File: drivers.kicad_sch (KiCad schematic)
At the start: 61 parts, among them J12 Conn_01x06_Female, Q1 FQP30N06, Q2 FQP30N06, Q3 FQP30N06, Q4 FQP30N06, Q5 FQP30N06, Q6 FQP30N06

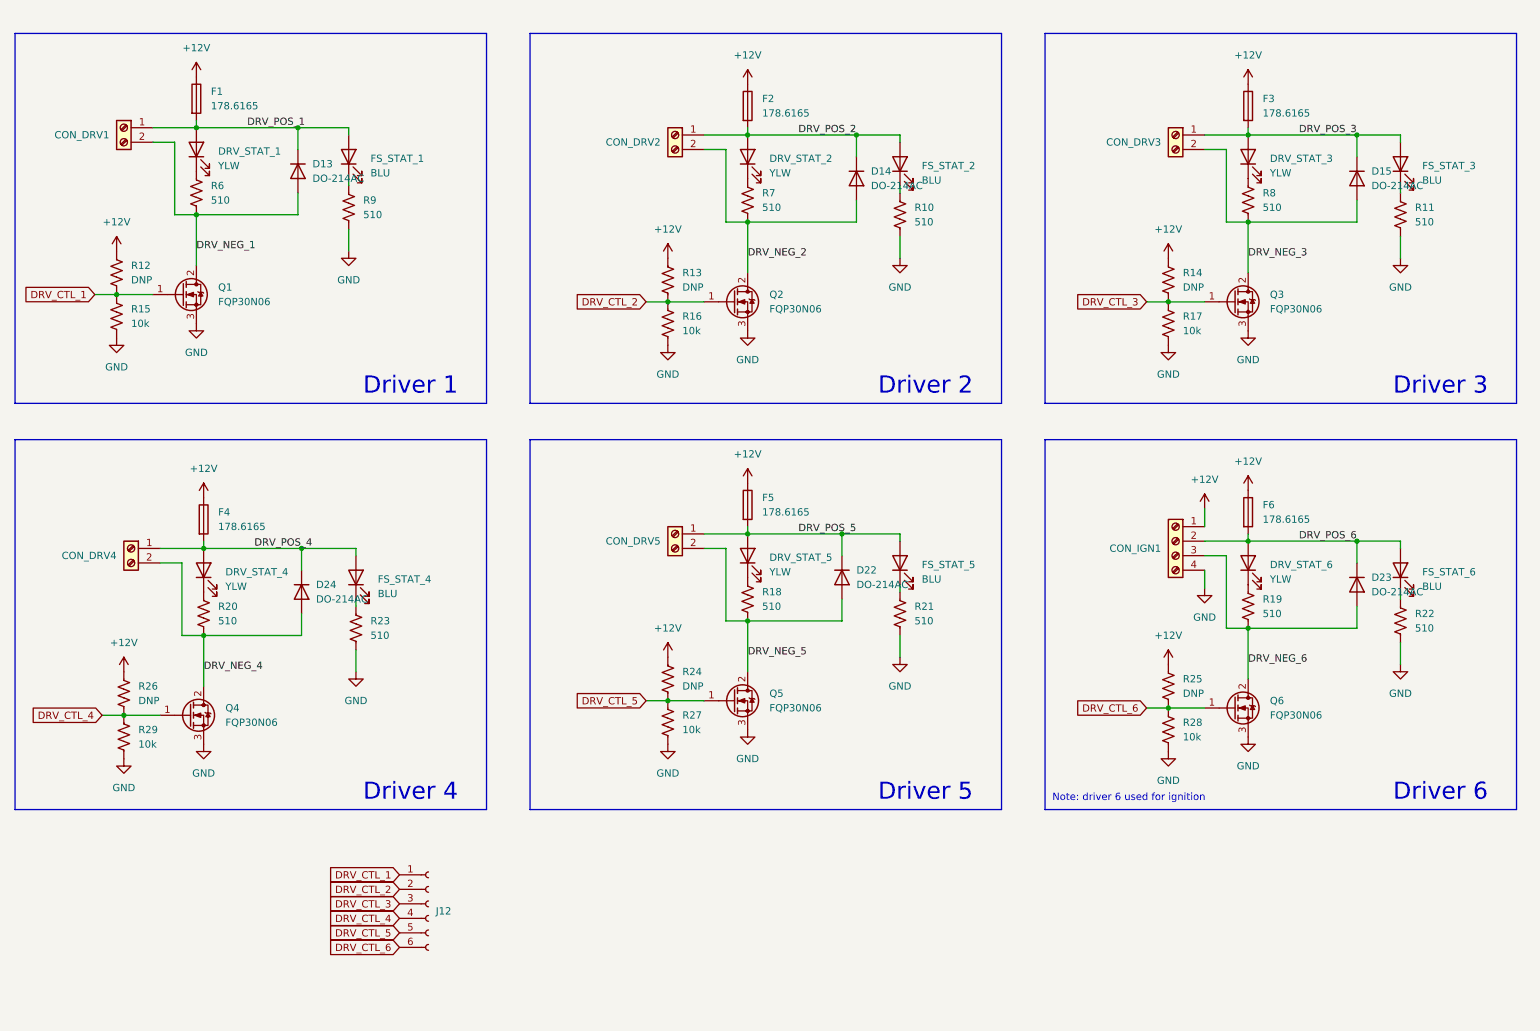
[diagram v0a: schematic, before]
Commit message: done schematiccing after design review
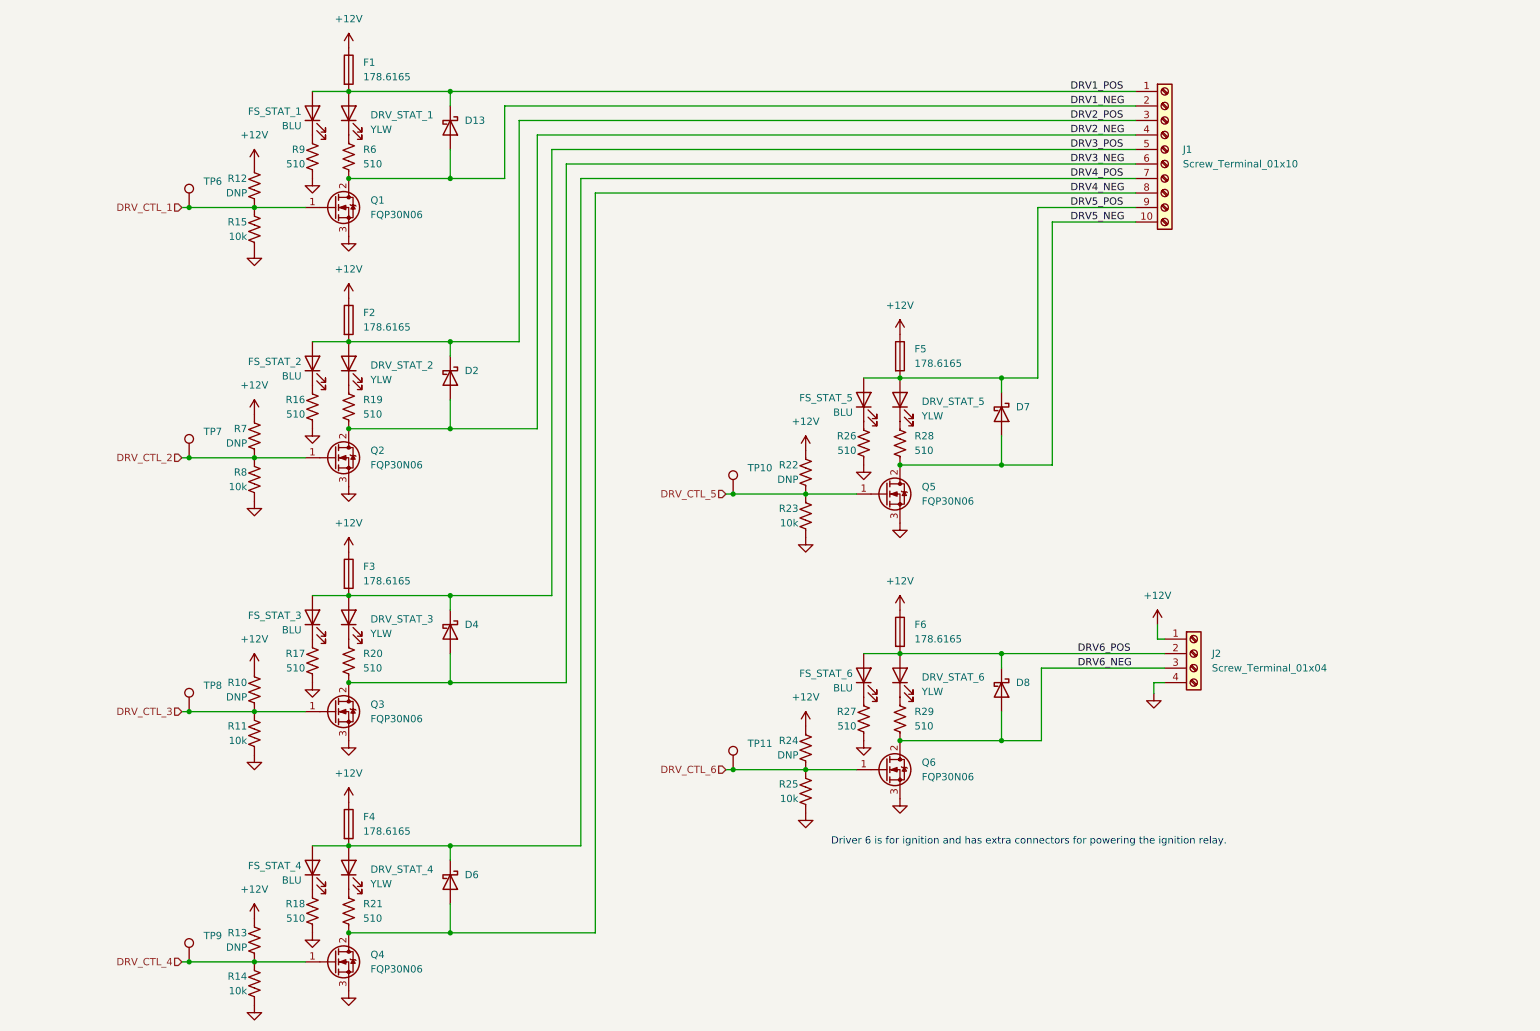
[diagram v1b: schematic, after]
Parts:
- removed CON_DRV1, CON_DRV2, CON_DRV3, CON_DRV4, CON_DRV5: Screw_Terminal_01x02, 1190363:1190363, symbol Connector:Screw_Terminal_01x02
- removed CON_IGN1: Screw_Terminal_01x02, 1190365:1190365, symbol Connector:Screw_Terminal_01x04
- removed D14, D15, D22, D23, D24: DO-214AC, karca_custom_footprints:DO-214AC, symbol Device:D
- removed J12: Conn_01x06_Female, Connector_PinSocket_2.54mm:PinSocket_1x06_P2.54mm_Vertical, symbol Connector:Conn_01x06_Female
- added D2, D4, D6, D7, D8: CDBA340-HF, Diode_SMD:D_SMA, symbol Device:D_Schottky
- added J1: Screw_Terminal_01x10, symbol Connector:Screw_Terminal_01x10
- added J2: Screw_Terminal_01x04, symbol Connector:Screw_Terminal_01x04
- added TP10, TP11, TP6, TP7, TP8, TP9: TestPoint, symbol Connector:TestPoint
- D13: value DO-214AC -> CDBA340-HF; footprint karca_custom_footprints:DO-214AC -> Diode_SMD:D_SMA; symbol Device:D -> Device:D_Schottky
- R10, R22, R7: value 510 -> DNP
- R11, R23, R8: value 510 -> 10k
- R14, R25: value DNP -> 10k
- R16, R17, R27, R28, R29: value 10k -> 510
- R26: value DNP -> 510
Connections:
- net +12V: now also R10.1, R22.1, R7.1, J2.1 (Pin_1); no longer R14.1, R25.1, R26.1
- net DRV_CTL_1: now also TP6.1
- net DRV_CTL_2: now also R7.2, R8.1, TP7.1; no longer R13.2, R16.1
- net DRV_CTL_3: now also R10.2, R11.1, TP8.1; no longer R14.2, R17.1
- net DRV_CTL_4: now also R13.2, R14.1, TP9.1; no longer R26.2, R29.1
- net DRV_CTL_5: now also R22.2, R23.1, TP10.1; no longer R24.2, R27.1
- net DRV_CTL_6: now also R24.2, R25.1, TP11.1; no longer R25.2, R28.1
- net GND: now also R14.2, R18.2, R25.2, R26.2, R8.2, J2.4 (Pin_4); no longer R10.2, R21.2, R22.2, R28.2, R29.2
- net at DRV_STAT_3.1 (K): now also R20.1; no longer R8.1
- net at FS_STAT_3.1 (K): now also R17.1; no longer R11.1
- net at R18.1: now also FS_STAT_4.1 (K); no longer DRV_STAT_5.1 (K)
- net at DRV_STAT_2.1 (K): now also R19.1; no longer R7.1
- net at FS_STAT_5.1 (K): now also R26.1; no longer R21.1
- net at DRV_STAT_6.1 (K): now also R29.1; no longer R19.1
- net at FS_STAT_6.1 (K): now also R27.1; no longer R22.1
- net at FS_STAT_2.1 (K): now also R16.1; no longer R10.1
- net at DRV_STAT_4.1 (K): now also R21.1; no longer R20.1
- net DRV_NEG_1 renamed DRV1_NEG
- net DRV1_NEG: now also J1.2 (Pin_2)
- net DRV_NEG_2 renamed DRV2_NEG
- net DRV2_NEG: now also R19.2, D2.2 (A), J1.4 (Pin_4); no longer R7.2
- net DRV_NEG_3 renamed DRV3_NEG
- net DRV3_NEG: now also R20.2, D4.2 (A), J1.6 (Pin_6); no longer R8.2
- net DRV_NEG_4 renamed DRV4_NEG
- net DRV4_NEG: now also R21.2, D6.2 (A), J1.8 (Pin_8); no longer R20.2
- net DRV_NEG_5 renamed DRV5_NEG
- net DRV5_NEG: now also R28.2, D7.2 (A), J1.10 (Pin_10); no longer R18.2
- net DRV_NEG_6 renamed DRV6_NEG
- net DRV6_NEG: now also R29.2, D8.2 (A), J2.3 (Pin_3); no longer R19.2
- net DRV_POS_1 renamed DRV1_POS
- net DRV1_POS: now also J1.1 (Pin_1)
- net DRV_POS_2 renamed DRV2_POS
- net DRV2_POS: now also D2.1 (K), J1.3 (Pin_3)
- net DRV_POS_3 renamed DRV3_POS
- net DRV3_POS: now also D4.1 (K), J1.5 (Pin_5)
- net DRV_POS_4 renamed DRV4_POS
- net DRV4_POS: now also D6.1 (K), J1.7 (Pin_7)
- net DRV_POS_5 renamed DRV5_POS
- net DRV5_POS: now also D7.1 (K), J1.9 (Pin_9)
- net DRV_POS_6 renamed DRV6_POS
- net DRV6_POS: now also D8.1 (K), J2.2 (Pin_2)
- new net: DRV_STAT_5.1 (K), R28.1
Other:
- note added: "Driver 6 is for ignition and has extra connectors for powering the ignition relay."
- note removed: "Driver 1"
- note removed: "Driver 2"
- note removed: "Driver 3"
- note removed: "Driver 4"
- note removed: "Driver 5"
- note removed: "Driver 6"
- note removed: "Note: driver 6 used for ignition"
- moved on the sheet: D13, DRV_STAT_1, F1, FS_STAT_1, Q1, R12, R15, R6, R9

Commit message: cleaned up PT footprint
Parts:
- J2: footprint (none) -> 1190365:1190365
- TP10, TP11, TP6, TP7, TP8, TP9: footprint (none) -> TestPoint:TestPoint_Pad_D2.0mm
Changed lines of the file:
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@@
       (effects (font (size 1.27 1.27)) (justify left) hide)
     )
-    (property "Footprint" "" (id 2) (at 52.07 179.07 0)
+    (property "Footprint" "TestPoint:TestPoint_Pad_D2.0mm" (id 2) (at 52.07 179.07 0)
       (effects (font (size 1.27 1.27)) hide)
     )
@@
       (effects (font (size 1.27 1.27)) (justify left) hide)
     )
-    (property "Footprint" "" (id 2) (at 147.32 97.155 0)
+    (property "Footprint" "TestPoint:TestPoint_Pad_D2.0mm" (id 2) (at 147.32 97.155 0)
       (effects (font (size 1.27 1.27)) hide)
     )
@@
       (effects (font (size 1.27 1.27)) (justify left) hide)
     )
-    (property "Footprint" "" (id 2) (at 52.07 135.255 0)
+    (property "Footprint" "TestPoint:TestPoint_Pad_D2.0mm" (id 2) (at 52.07 135.255 0)
       (effects (font (size 1.27 1.27)) hide)
     )
@@
       (effects (font (size 1.27 1.27)) (justify left) hide)
     )
-    (property "Footprint" "" (id 2) (at 147.32 145.415 0)
+    (property "Footprint" "TestPoint:TestPoint_Pad_D2.0mm" (id 2) (at 147.32 145.415 0)
       (effects (font (size 1.27 1.27)) hide)
     )
@@
       (effects (font (size 1.27 1.27)) (justify left) hide)
     )
-    (property "Footprint" "" (id 2) (at 52.07 90.805 0)
+    (property "Footprint" "TestPoint:TestPoint_Pad_D2.0mm" (id 2) (at 52.07 90.805 0)
       (effects (font (size 1.27 1.27)) hide)
     )
@@
       (effects (font (size 1.27 1.27)) (justify left) hide)
     )
-    (property "Footprint" "" (id 2) (at 52.07 46.99 0)
+    (property "Footprint" "TestPoint:TestPoint_Pad_D2.0mm" (id 2) (at 52.07 46.99 0)
       (effects (font (size 1.27 1.27)) hide)
     )
@@
       (effects (font (size 1.27 1.27)) (justify left))
     )
-    (property "Footprint" "" (id 2) (at 222.885 125.095 0)
-      (effects (font (size 1.27 1.27)) hide)
-    )
+    (property "Footprint" "1190365:1190365" (id 2) (at 222.885 125.095 0)
+      (effects (font (size 1.27 1.27)) hide)
+    )
